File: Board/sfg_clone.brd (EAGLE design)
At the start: 134 x 121 mm, 121 parts, among them IC1 27C512AP, IC2 74LS04D, IC3 EPM7160-T100, IC4 YM2151, IC5 YM3012, IC6 LM4556N, IC7 LM4556N, IC8 LM4558N, IC9 TLP552, Q1 4mHz, T1 2SC1815, T2 BC637, T3 BC637, T4 BC637, T5 BC557A, T6 BC548A, X1 SFG-60, X2 SFG-20, X3 MIDI_CONN_FEMALE_SUPPORT, X4 MIDI_CONN_FEMALE_SUPPORT, X5 RCA, X6 RCA, X7 JTAG10, X8A AUDIO, X8B AUDIO

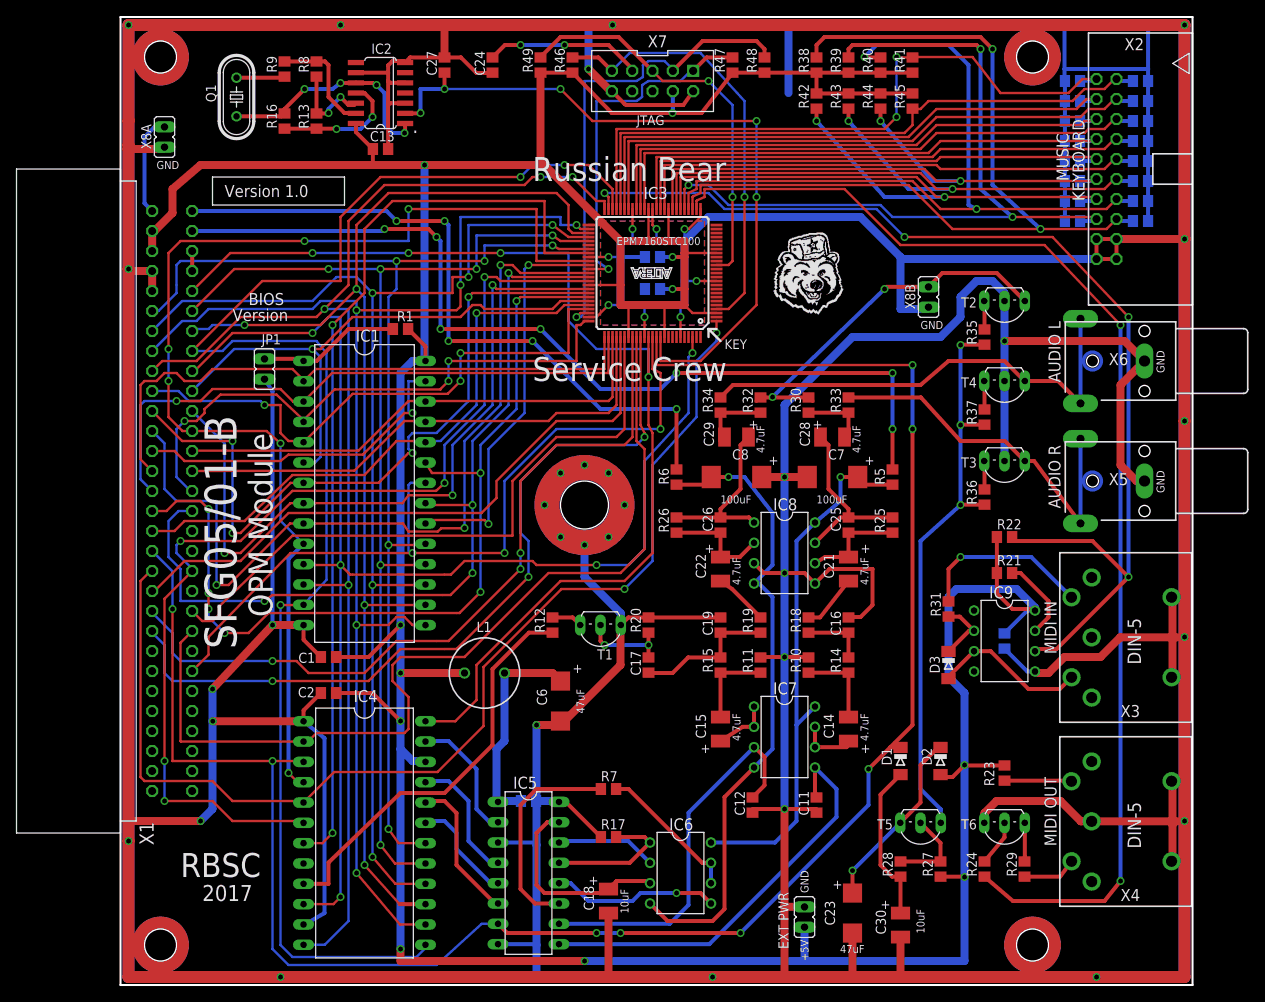
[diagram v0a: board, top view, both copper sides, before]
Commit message: Board updated to version 1.1
Board updated to version 1.1
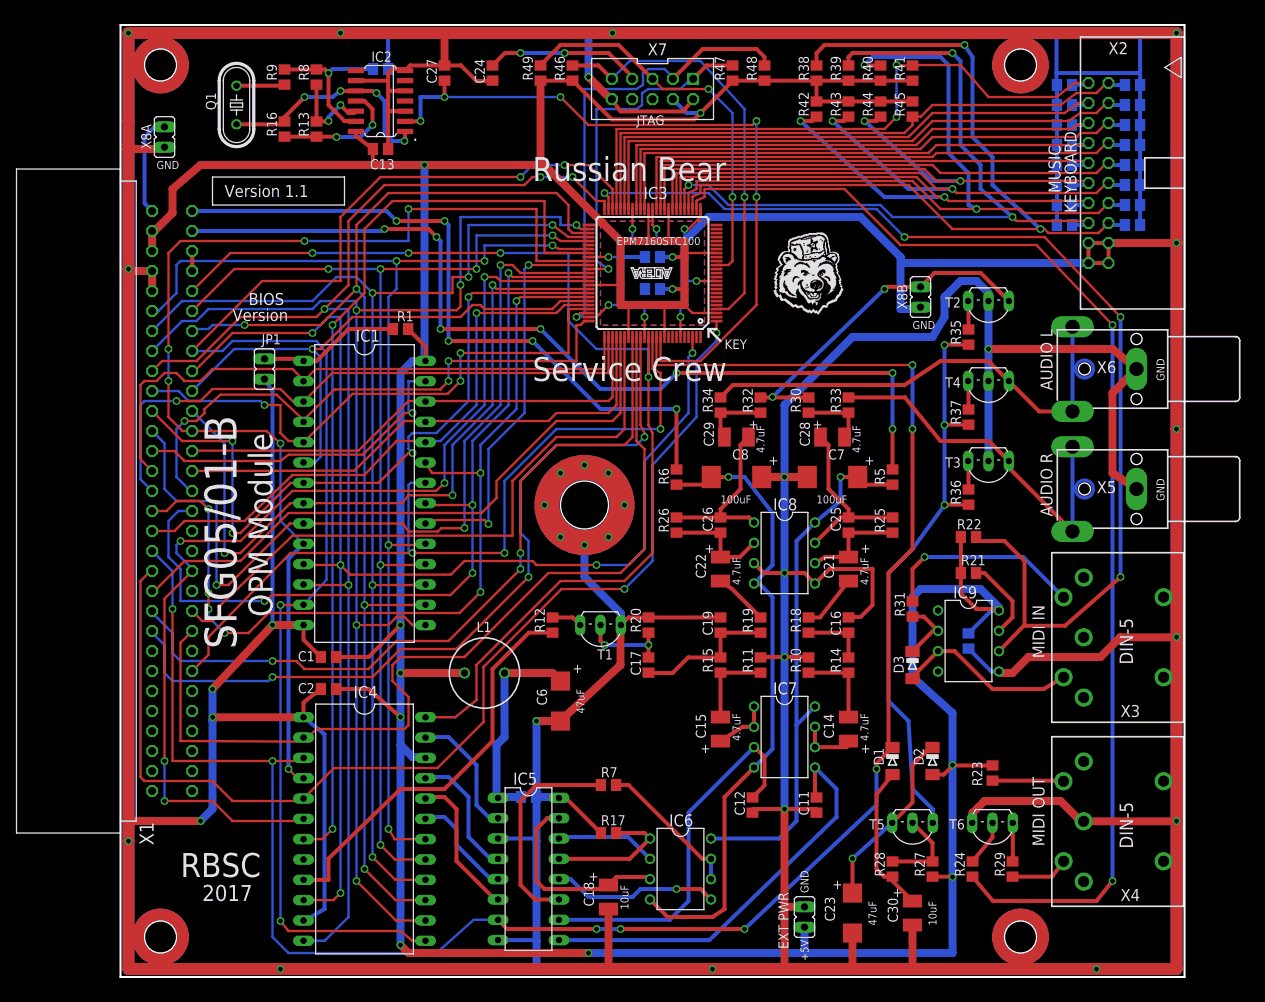
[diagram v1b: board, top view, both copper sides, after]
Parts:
- added C3: 47pF, rcl:C0805
- moved C20 4.50 mm to (106.0, 43.0)
- moved D3 4.50 mm to (99.0, 40.0)
- moved IC9 4.50 mm to (106.0, 43.0)
- moved R21 4.50 mm to (106.0, 51.5)
- moved R22 4.50 mm to (106.0, 56.0)
- moved R31 4.50 mm to (99.0, 47.0)
- moved C30 2.12 mm to (99.0, 9.00)
- moved R35 2.00 mm to (106.0, 81.0)
- moved R36 2.00 mm to (106.0, 61.0)
- moved R37 2.00 mm to (106.0, 71.0)
- moved T2 2.00 mm to (108.5, 85.5)
- moved T3 2.00 mm to (108.5, 65.5)
- moved T4 2.00 mm to (108.5, 75.5)
- moved R23 1.50 mm to (109.0, 26.5)
- moved R24 1.50 mm to (106.5, 14.5)
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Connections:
- net GND: now also C3.2
- net N$8: now also C3.1
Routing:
- net GND: track 1878.0 -> 1842.1 mm
- net N$8: track 14.0 -> 19.7 mm, vias 0 -> 1
- net +5V: track 525.7 -> 520.1 mm
- net SD1: track 98.9 -> 95.4 mm
- net N$27: track 22.1 -> 25.6 mm
- net D2: track 186.2 -> 182.8 mm, vias 3 -> 4
- net N$26: track 19.5 -> 22.8 mm
- net SD2: track 96.2 -> 93.1 mm
- net SD0: track 110.4 -> 107.4 mm
- net SD3: track 83.2 -> 80.7 mm
- net RESET: track 246.2 -> 243.8 mm
- net N$4: track 46.7 -> 44.7 mm
- net SD7: track 77.7 -> 75.7 mm
- net N$64: track 72.1 -> 73.4 mm
- net ST0: track 72.1 -> 70.8 mm
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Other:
- board size 134 x 121 mm -> 133 x 119 mm
- board text added: "Optional. Use with 74HCT04"
- board text added: "Version 1.1"
- board text removed: "Version 1.0"
